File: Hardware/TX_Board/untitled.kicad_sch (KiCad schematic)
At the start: 42 parts, among them IC7 MAPS-010164-TR0500, IC8 QPA9122TR7, J13 MM8030-2610RJ3, J14 MM8030-2610RJ3, J15 Conn_Coaxial

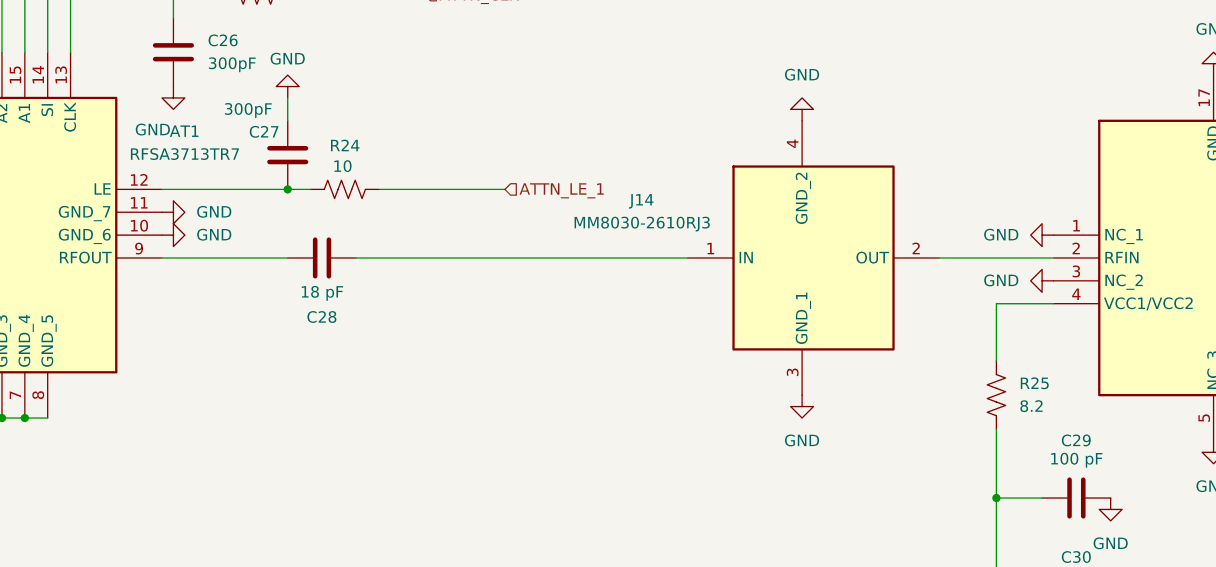
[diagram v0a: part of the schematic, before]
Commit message: Updated Layout
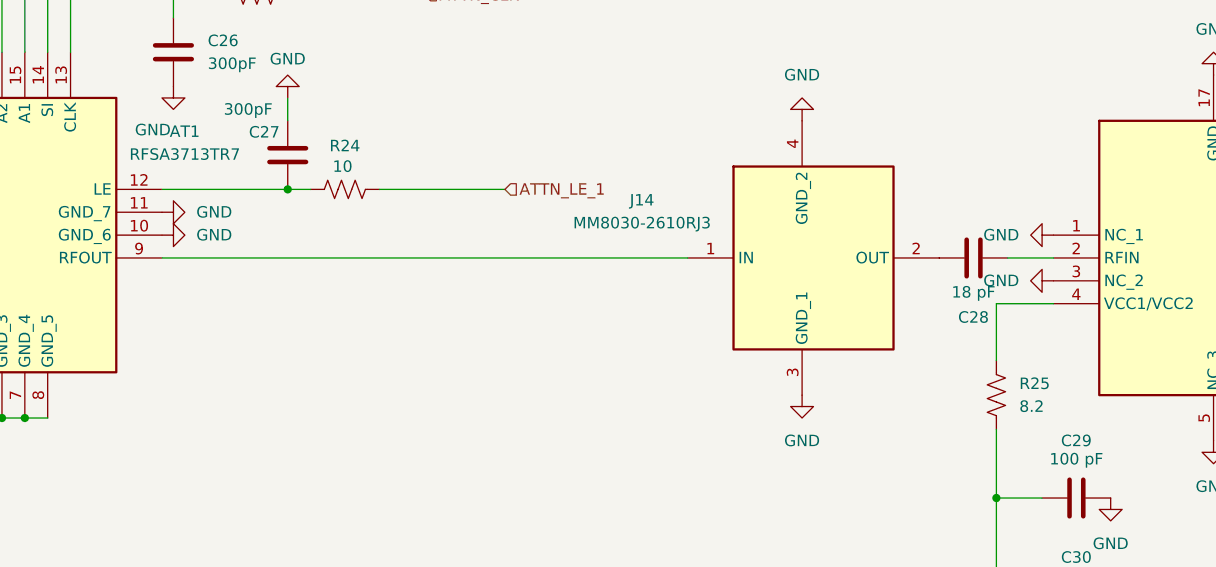
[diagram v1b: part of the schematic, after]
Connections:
- net at IC8.2 (RFIN): now also C28.2; no longer J14.2 (OUT)
- net at C28.1: now also J14.2 (OUT); no longer AT1.9 (RFOUT)
- net at J14.1 (IN): now also AT1.9 (RFOUT); no longer C28.2
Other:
- moved on the sheet: C28
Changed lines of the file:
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@@
 	(wire
 		(pts
-			(xy 229.87 151.13) (xy 266.7 151.13)
-		)
-		(stroke
-			(width 0)
-			(type default)
-		)
-	)
-	(wire
-		(pts
 			(xy 335.28 107.95) (xy 335.28 92.71)
 		)
@@
 	(wire
 		(pts
-			(xy 294.64 151.13) (xy 307.34 151.13)
-		)
-		(stroke
-			(width 0)
-			(type default)
-		)
-	)
-	(wire
-		(pts
 			(xy 222.25 133.35) (xy 222.25 135.89)
 		)
@@
 	(wire
 		(pts
-			(xy 208.28 151.13) (xy 222.25 151.13)
+			(xy 167.64 143.51) (xy 177.8 143.51)
 		)
 		(stroke
@@
 	(wire
 		(pts
-			(xy 167.64 143.51) (xy 177.8 143.51)
+			(xy 49.53 151.13) (xy 58.42 151.13)
 		)
 		(stroke
@@
 	(wire
 		(pts
-			(xy 49.53 151.13) (xy 58.42 151.13)
+			(xy 208.28 151.13) (xy 266.7 151.13)
 		)
 		(stroke
@@
 	(wire
 		(pts
+			(xy 302.26 151.13) (xy 307.34 151.13)
+		)
+		(stroke
+			(width 0)
+			(type default)
+		)
+	)
+	(wire
+		(pts
 			(xy 187.96 168.91) (xy 187.96 172.72)
 		)
@@
 	(symbol
 		(lib_id "tx_board_symbol_library:C")
-		(at 226.06 151.13 90)
+		(at 298.45 151.13 90)
 		(unit 1)
 		(exclude_from_sim no)
@@
 		(dnp no)
 		(property "Reference" "C28"
-			(at 226.06 157.734 90)
+			(at 298.45 157.734 90)
 			(effects
 				(font
@@
 		)
 		(property "Value" "18 pF"
-			(at 226.06 154.94 90)
+			(at 298.45 154.94 90)
 			(effects
 				(font
@@
 		)
 		(property "Footprint" "Capacitor_SMD:C_0402_1005Metric"
-			(at 229.87 150.1648 0)
+			(at 302.26 150.1648 0)
 			(effects
 				(font
@@
 		)
 		(property "Datasheet" "~"
-			(at 226.06 151.13 0)
+			(at 298.45 151.13 0)
 			(effects
 				(font
@@
 		)
 		(property "Description" "Unpolarized capacitor"
-			(at 226.06 151.13 0)
+			(at 298.45 151.13 0)
 			(effects
 				(font
